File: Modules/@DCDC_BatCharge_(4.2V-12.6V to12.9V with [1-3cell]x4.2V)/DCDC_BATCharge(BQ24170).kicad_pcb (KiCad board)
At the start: 2 copper layers, 44 x 40.2 mm, 88 parts, among them J1 Btn_LED, J2 VIA_V_PACK, J3 VIA_GND, J4 VIA_V_Adapter, J5 VIA_V_SYS, Q1 AO3416, Q2 AO3416, Q3 AO3415, U1 BQ24170, U2 TPS61288, U3 TPS61288

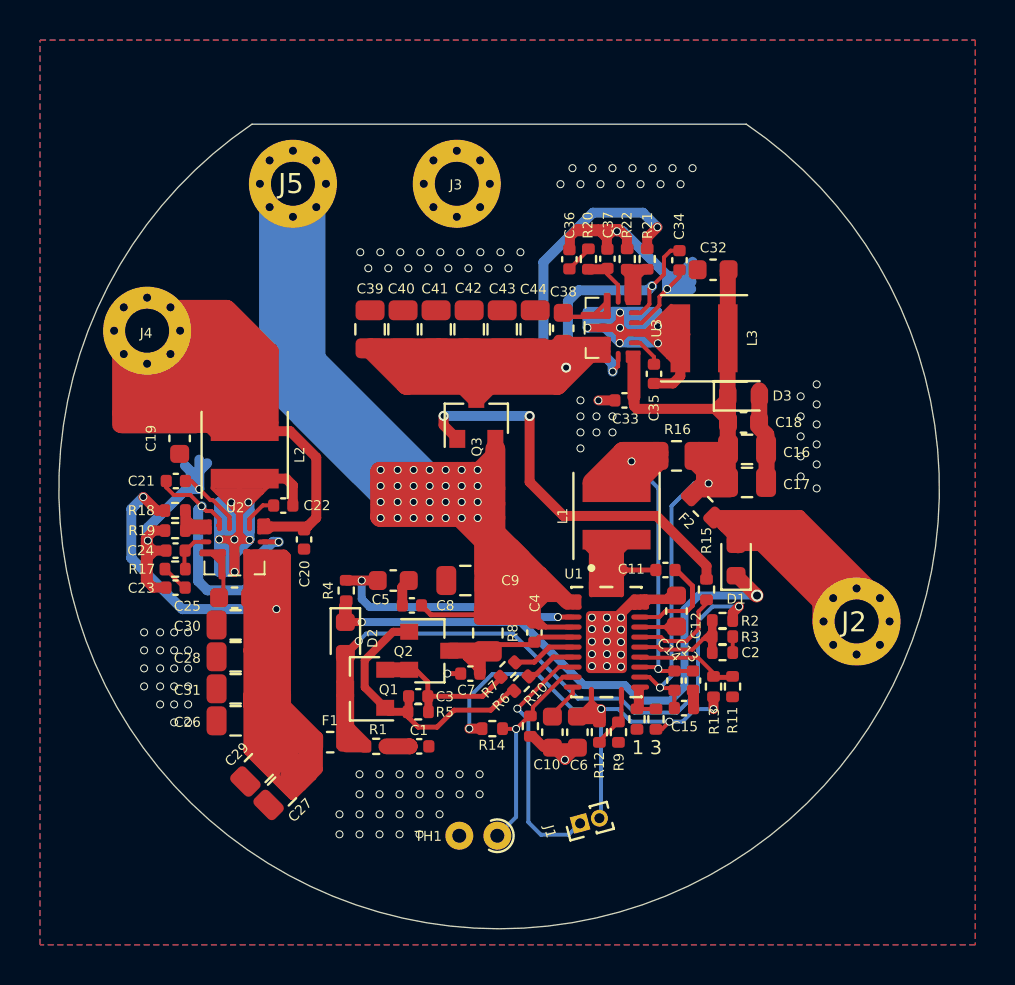
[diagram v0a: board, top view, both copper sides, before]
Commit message: Sort Out
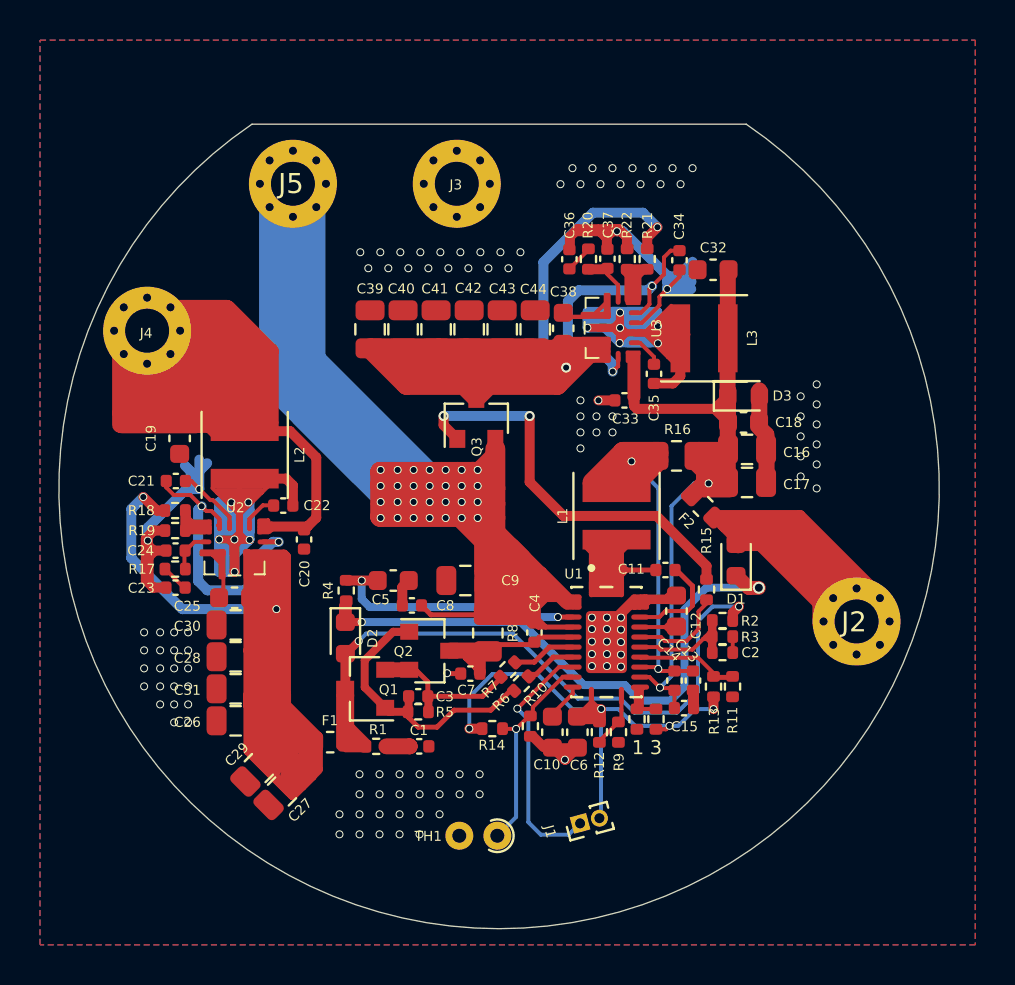
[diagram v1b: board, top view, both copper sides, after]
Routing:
- net Net-(D2-Pad2): track 53.0 -> 48.4 mm
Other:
- net class Default removed
